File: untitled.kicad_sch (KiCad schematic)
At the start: 21 parts, among them IC10 ILD206T, IC12 ILD206T, IC2 ILD206T, IC3 ILD206T, IC4 ILD206T, IC5 ILD206T, IC6 ILD206T, IC7 ILD206T, IC8 ILD206T, IC9 ILD206T, J2 1147330000, J3 1147330000, J4 1147330000, K1 G2RL-1-H, U2 5-1415390-1, U3 5-1415390-1, U4 5-1415390-1

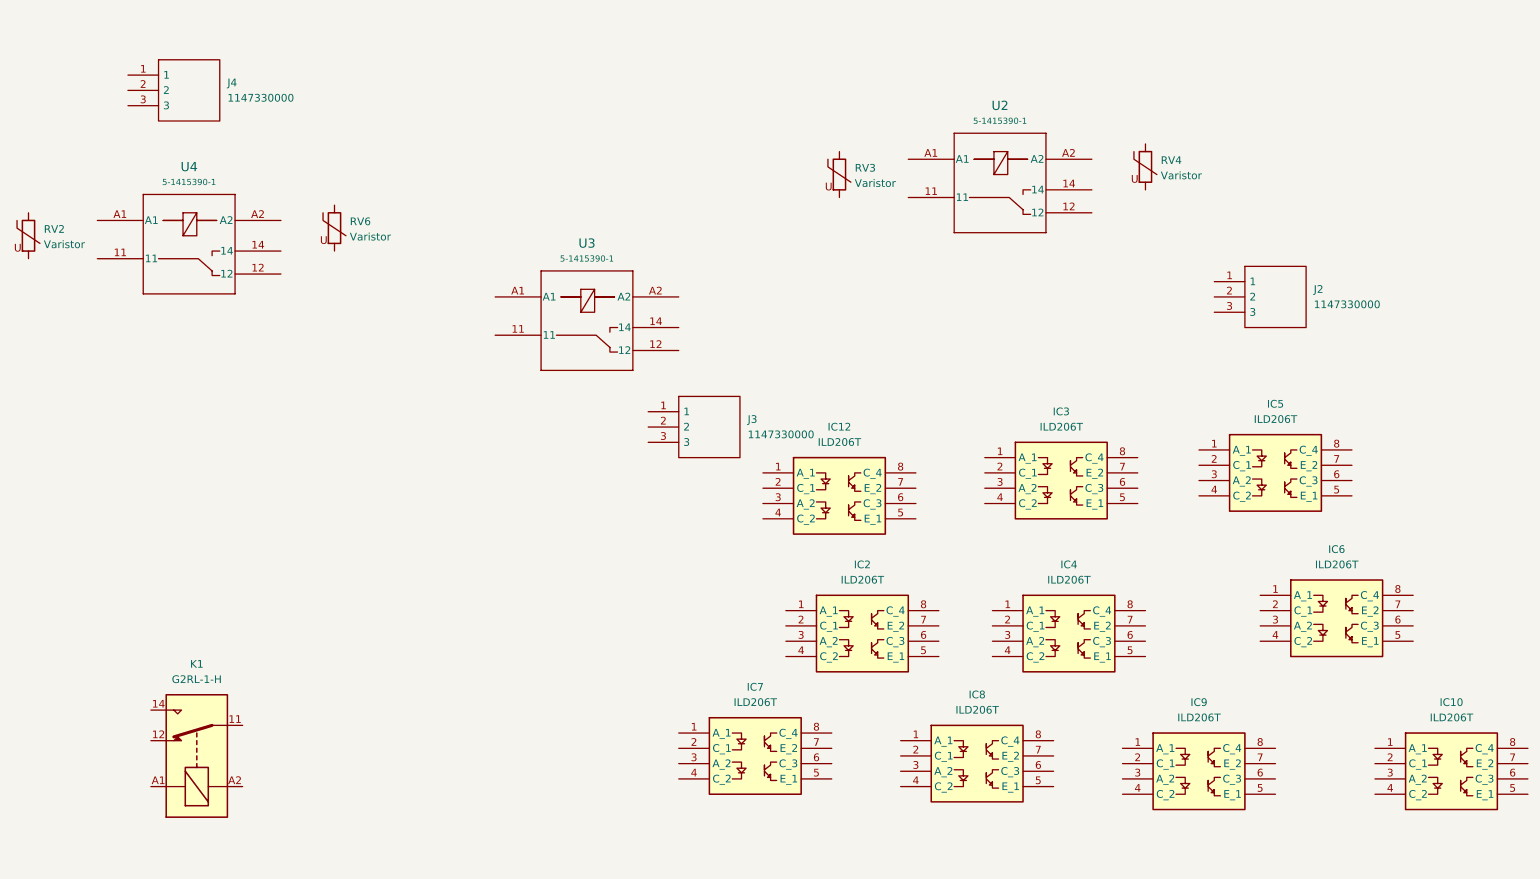
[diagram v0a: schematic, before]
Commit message: 7-mayo-2026 831am
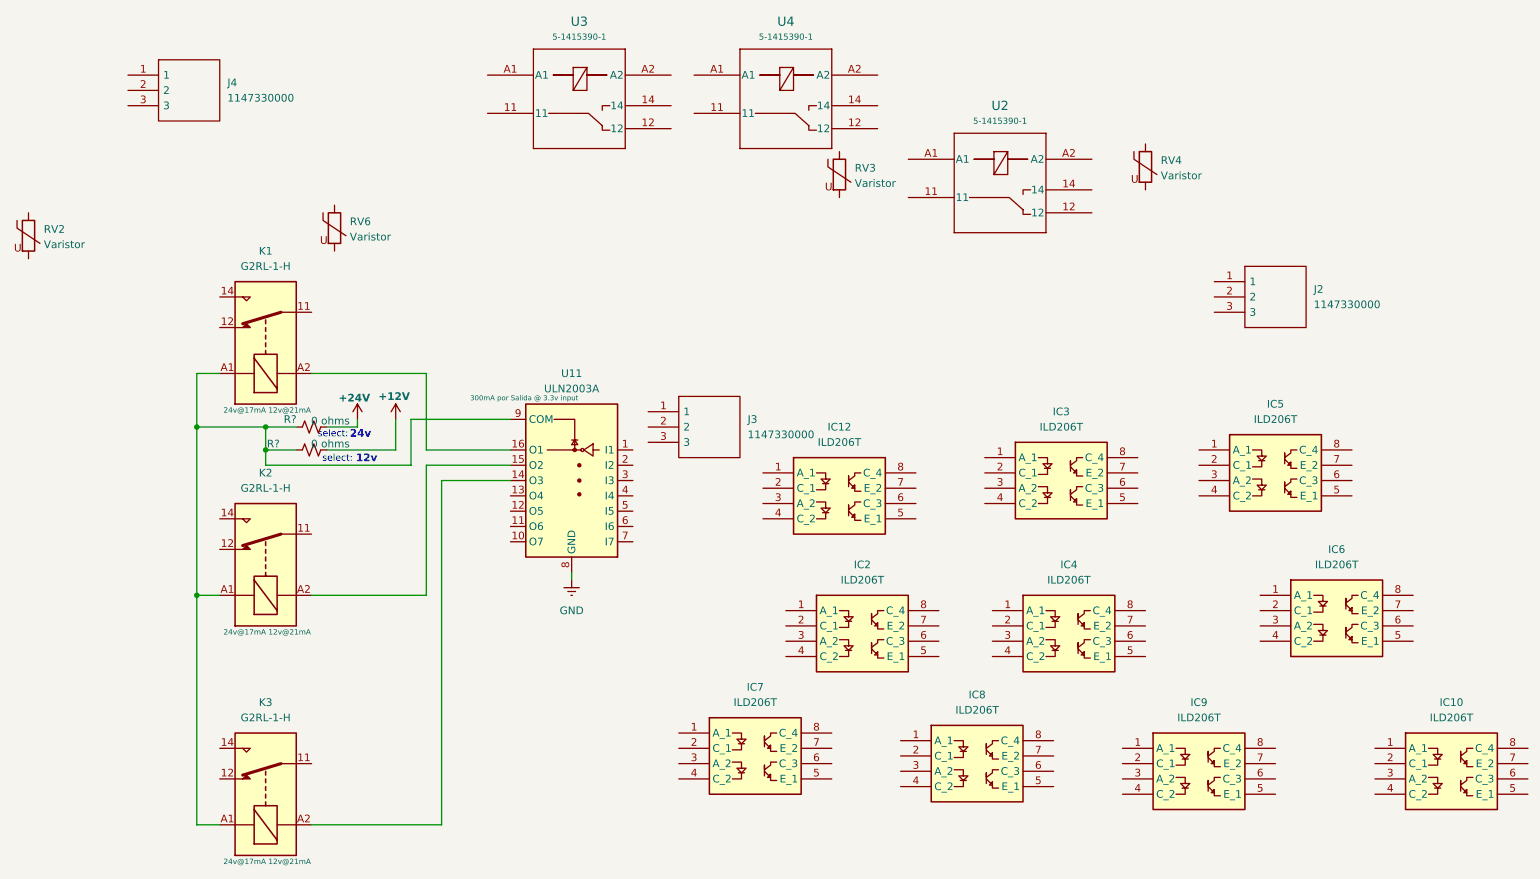
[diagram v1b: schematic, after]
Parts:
- added K2, K3: G2RL-1-H, Relay_THT:Relay_SPDT_Omron_G2RL-1, symbol Relay:G2RL-1-H
- added R? (x2): 0 ohms, symbol Device:R_Small_US
- added U11: ULN2003A, symbol Transistor_Array:ULN2003A
- K1: corriente  (none) -> 24v@17mA 12v@21mA
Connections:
- net at K1.A1: now also K2.A1, K3.A1, R?.1, R?.1, U11.9 (COM)
- net at K1.A2: now also U11.16 (O1)
- new net: K3.A2, U11.14 (O3)
- new net: K2.A2, U11.15 (O2)
- new net +12V: R?.2
- new net +24V: R?.2
- new net GND: U11.8 (GND)
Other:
- note added: "12v"
- note added: "24v"
- note added: "select:"
- moved on the sheet: K1, U3, U4
